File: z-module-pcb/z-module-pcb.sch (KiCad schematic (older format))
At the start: 29 parts, among them K1 RELAY_VAC_VAC, K2 RELAY_VAC_EJECT, K3 REL_VAC_SENSE, P1 STEP_Z, P2 STEP_A, P3 CONTROL, P4 PWR, P5 MOT_Z, P6 MOT_A, P7 VADMI, P8 LED, P9 LIMIT_SWS, U1 4N25, U2 4N25, U3 4N25, U4 LDD300, U5 SilentStepStick, U6 SilentStepStick

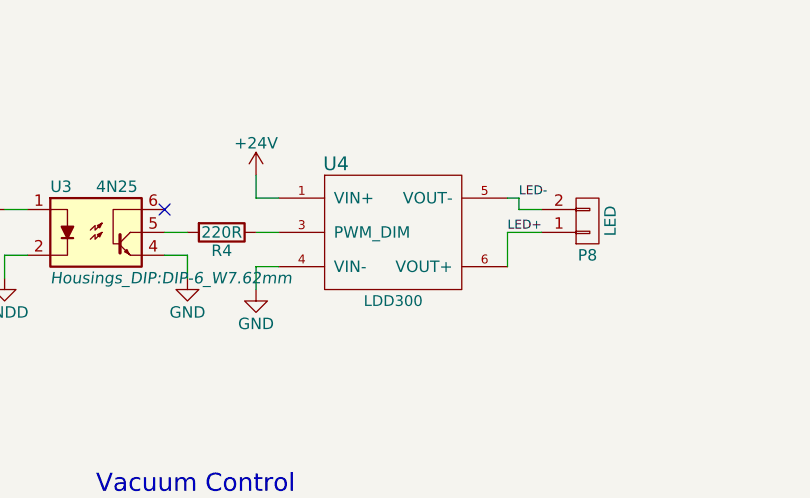
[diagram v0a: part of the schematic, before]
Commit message: Finalized and cleaned design
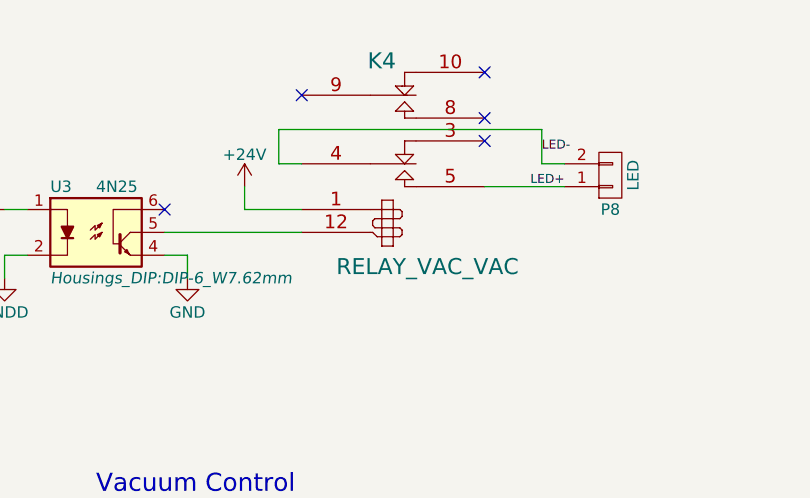
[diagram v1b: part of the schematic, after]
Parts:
- removed R4: 220R, Resistors_ThroughHole:Resistor_Horizontal_RM10mm, symbol R
- removed U4: LDD300, z-module-pcb:Meanwell_LDD300, symbol LDD300
- added K4: RELAY_VAC_VAC, z-module-pcb:AxicomRelay-V23079, symbol RELAY_AXICOM_V23079
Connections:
- net +24V: now also K4.1
- net LED+: now also K4.5
- net LED-: now also K4.4
- net at U3.5: now also K4.12
- no-connect marks 22 -> 26
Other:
- moved on the sheet: P8
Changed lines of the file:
@@
 L CONN_01X02 P8
 U 1 1 5640EF0F
-P 6850 1750
-F 0 "P8" H 6850 1900 50  0000 C CNN
-F 1 "LED" V 6950 1750 50  0000 C CNN
-F 2 "z-module-pcb:AKL_182-02" H 6850 1750 60  0001 C CNN
-F 3 "" H 6850 1750 60  0000 C CNN
-	1    6850 1750
+P 6950 1550
+F 0 "P8" H 6950 1700 50  0000 C CNN
+F 1 "LED" V 7050 1550 50  0000 C CNN
+F 2 "z-module-pcb:AKL_182-02" H 6950 1550 60  0001 C CNN
+F 3 "" H 6950 1550 60  0000 C CNN
+	1    6950 1550
 	1    0    0    1
 $EndComp
@@
 Wire Wire Line
 	3900 1700 4000 1700
-$Comp
-L LDD300 U4
-U 1 1 5641EE6C
-P 6000 1800
-F 0 "U4" H 5750 2100 60  0000 C CNN
-F 1 "LDD300" H 6000 1500 47  0000 C CNN
-F 2 "z-module-pcb:Meanwell_LDD300" H 6000 1400 60  0001 C CNN
-F 3 "" H 6000 1400 60  0000 C CNN
-	1    6000 1800
-	1    0    0    -1
-$EndComp
-Wire Wire Line
-	6500 1950 6500 1800
-Wire Wire Line
-	6500 1800 6650 1800
-Wire Wire Line
-	6650 1700 6550 1700
-Wire Wire Line
-	6550 1700 6550 1650
-Wire Wire Line
-	6550 1650 6500 1650
+Wire Wire Line
+	6400 1600 6750 1600
+Wire Wire Line
+	6650 1500 6750 1500
+Wire Wire Line
+	6650 1350 6650 1500
 $Comp
 L +3.3V #PWR028
@@
 	1    0    0    -1
 $EndComp
-$Comp
-L R R4
-U 1 1 5642067F
-P 5250 1800
-F 0 "R4" V 5330 1800 50  0000 C CNN
-F 1 "220R" V 5250 1800 50  0000 C CNN
-F 2 "Resistors_ThroughHole:Resistor_Horizontal_RM10mm" V 5180 1800 30  0001 C CNN
-F 3 "" H 5250 1800 30  0000 C CNN
-	1    5250 1800
-	0    1    1    0
-$EndComp
-Wire Wire Line
-	5000 1800 5100 1800
-Wire Wire Line
-	5400 1800 5500 1800
-$Comp
-L GND #PWR030
-U 1 1 56420906
-P 5400 2050
-F 0 "#PWR030" H 5400 1800 50  0001 C CNN
-F 1 "GND" H 5400 1900 50  0000 C CNN
-F 2 "" H 5400 2050 60  0000 C CNN
-F 3 "" H 5400 2050 60  0000 C CNN
-	1    5400 2050
-	1    0    0    -1
-$EndComp
-Wire Wire Line
-	5500 1950 5400 1950
-Wire Wire Line
-	5400 1950 5400 2050
-$Comp
-L +24V #PWR031
-U 1 1 56420C2E
-P 5400 1550
-F 0 "#PWR031" H 5400 1400 50  0001 C CNN
-F 1 "+24V" H 5400 1690 50  0000 C CNN
-F 2 "" H 5400 1550 60  0000 C CNN
-F 3 "" H 5400 1550 60  0000 C CNN
-	1    5400 1550
-	1    0    0    -1
-$EndComp
-Wire Wire Line
-	5400 1550 5400 1650
-Wire Wire Line
-	5400 1650 5500 1650
+Wire Wire Line
+	5000 1800 5600 1800
 Wire Wire Line
 	1500 5000 1700 5000
@@
 Wire Wire Line
 	9400 5550 9500 5550
-Text Label 6550 1650 0    39   ~ 0
+Text Label 6650 1450 0    39   ~ 0
 LED-
-Text Label 6500 1800 0    39   ~ 0
+Text Label 6600 1600 0    39   ~ 0
 LED+
 NoConn ~ 8750 1850
@@
 	0    1    1    0
 $EndComp
+$Comp
+L RELAY_AXICOM_V23079 K4
+U 1 1 56463762
+P 6000 1450
+F 0 "K4" H 5950 1850 70  0000 C CNN
+F 1 "RELAY_VAC_VAC" H 6150 950 70  0000 C CNN
+F 2 "z-module-pcb:AxicomRelay-V23079" H 6000 1450 60  0001 C CNN
+F 3 "" H 6000 1450 60  0000 C CNN
+F 4 "HFD3-024" H 6000 1450 60  0001 C CNN "Order"
+	1    6000 1450
+	1    0    0    -1
+$EndComp
+$Comp
+L +24V #PWR?
+U 1 1 5646376A
+P 5350 1600
+F 0 "#PWR?" H 5350 1450 50  0001 C CNN
+F 1 "+24V" H 5350 1740 50  0000 C CNN
+F 2 "" H 5350 1600 60  0000 C CNN
+F 3 "" H 5350 1600 60  0000 C CNN
+	1    5350 1600
+	1    0    0    -1
+$EndComp
+Wire Wire Line
+	5350 1600 5350 1700
+Wire Wire Line
+	5350 1700 5600 1700
+Wire Wire Line
+	5500 1500 5600 1500
+NoConn ~ 6400 1100
+NoConn ~ 6400 1300
+NoConn ~ 5600 1200
+Wire Wire Line
+	6650 1350 5500 1350
+Wire Wire Line
+	5500 1350 5500 1500
+NoConn ~ 6400 1400
 $EndSCHEMATC
